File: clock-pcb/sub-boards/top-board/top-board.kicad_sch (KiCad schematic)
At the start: 18 parts, among them J1 Conn_01x07_Socket, U1 BH1750FVI-TR, U3 OPT3004DTSR, U4 SHT4x

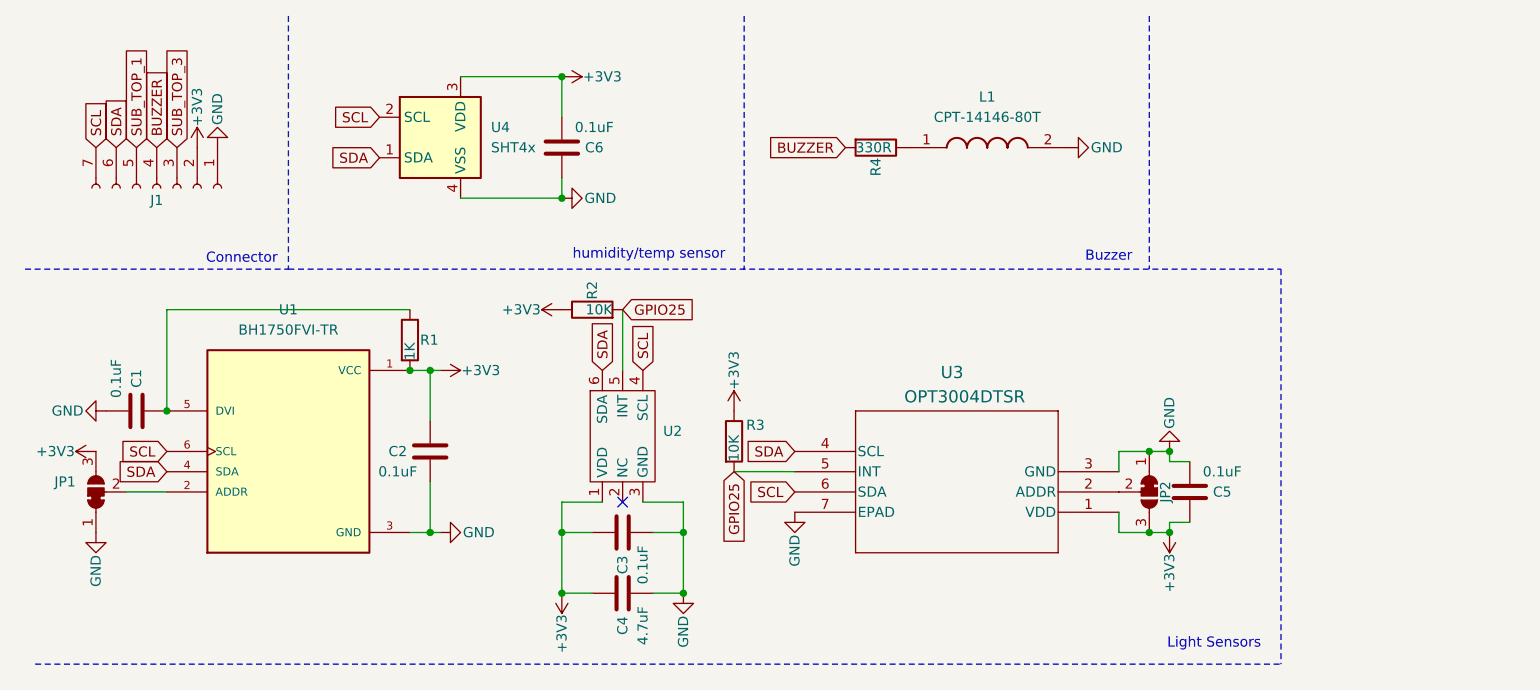
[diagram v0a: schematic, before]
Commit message: routing
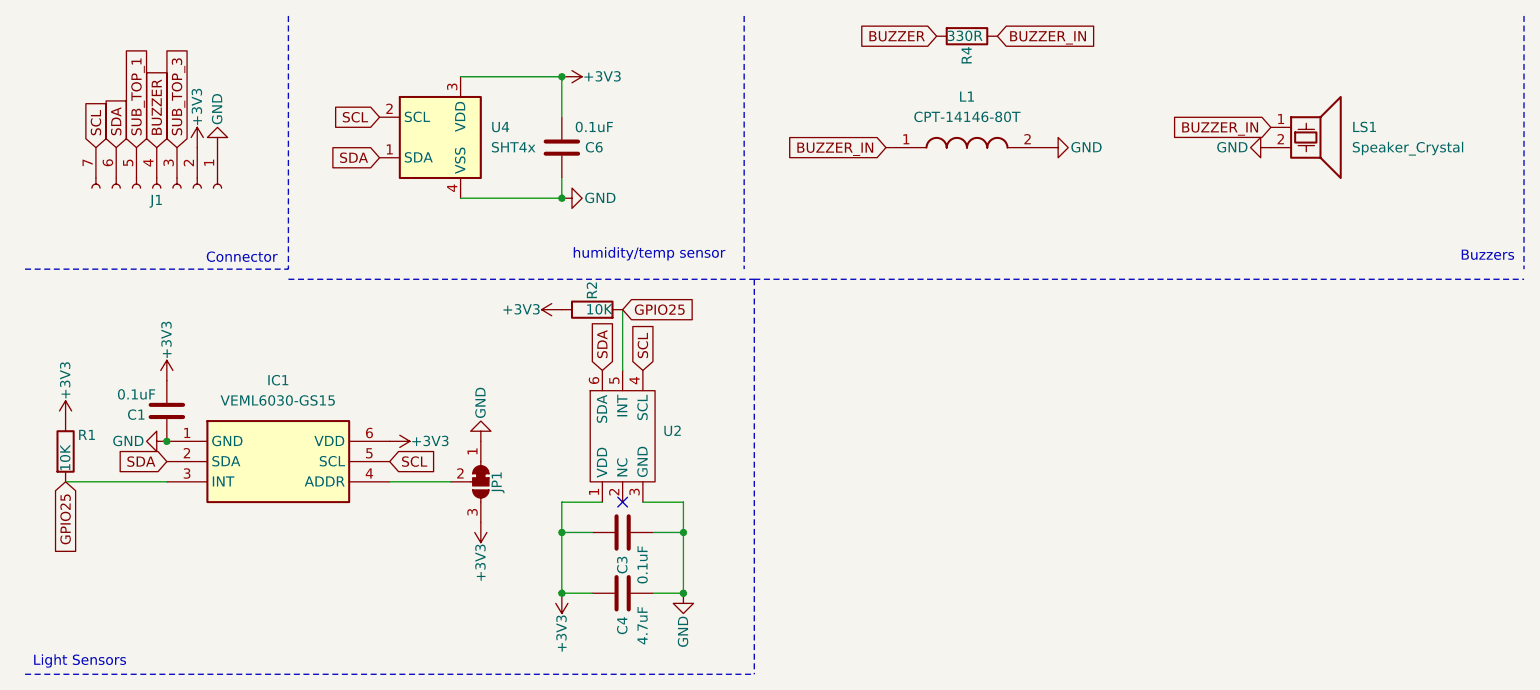
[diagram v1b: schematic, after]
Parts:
- removed C2, C5: 0.1uF, Capacitor_SMD:C_0603_1608Metric, symbol clock:C
- removed JP2: SolderJumper_3_Bridged12, Jumper:SolderJumper-3_P1.3mm_Bridged2Bar12_RoundedPad1.0x1.5mm, symbol clock:SolderJumper_3_Bridged12
- removed R3: 10K, Resistor_SMD:R_0402_1005Metric, symbol clock:R
- removed U1: BH1750FVI-TR, clock:XDCR_BH1750FVI-TR, symbol clock:BH1750FVI-TR
- removed U3: OPT3004DTSR, clock:DNP6_TEX, symbol clock:OPT3004DTSR
- added IC1: VEML6030-GS15, clock:VEML6030GS15, symbol VEML6030-GS15:VEML6030-GS15
- added LS1: Speaker_Crystal, clock:AST0760_MAL, symbol Device:Speaker_Crystal
- R1: value 1K -> 10K
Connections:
- net +3V3: now also C1.2, R1.1, IC1.6 (VDD); no longer R1.2
- net GND: now also C1.1, IC1.1 (GND), LS1.2; no longer C1.2
- net GPIO25: now also R1.2, IC1.3 (INT)
- net SCL: now also IC1.5 (SCL)
- net SDA: now also IC1.2 (SDA)
- net at JP1.2 (C): now also IC1.4 (ADDR)
- net BUZZER_IN: now reaches L1.1, R4.1
- net BUZZER_IN: now also LS1.1
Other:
- note added: "Buzzers"
- note removed: "Buzzer"
- moved on the sheet: L1, R4

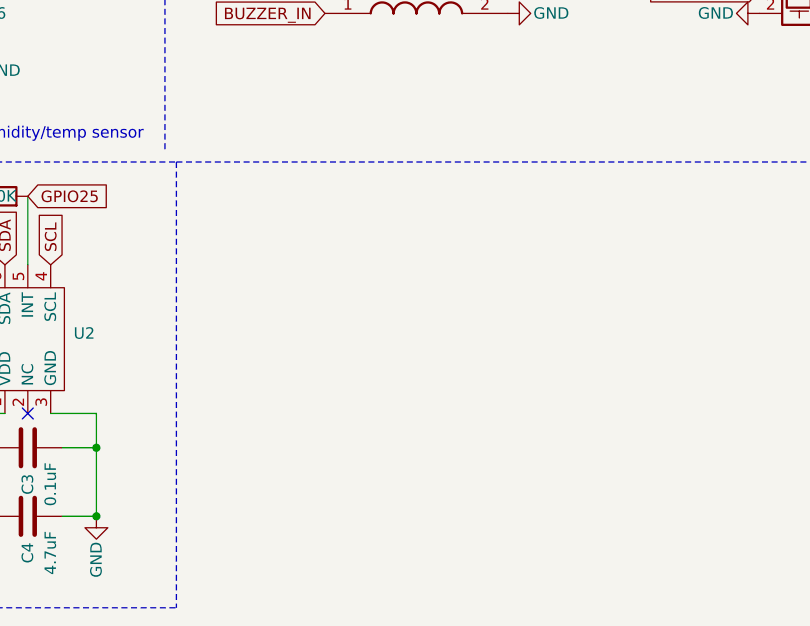
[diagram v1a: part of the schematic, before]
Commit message: touch slider pcb
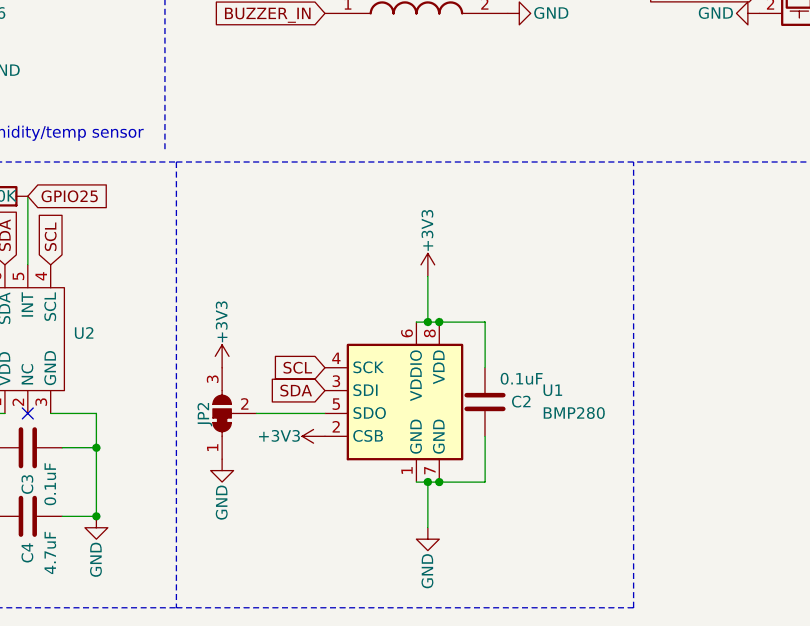
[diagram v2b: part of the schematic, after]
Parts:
- added C2: 0.1uF, Capacitor_SMD:C_0603_1608Metric, symbol clock:C
- added JP2: SolderJumper_3_Bridged12, Jumper:SolderJumper-3_P1.3mm_Bridged2Bar12_RoundedPad1.0x1.5mm, symbol clock:SolderJumper_3_Bridged12
- added U1: BMP280, Package_LGA:Bosch_LGA-8_2x2.5mm_P0.65mm_ClockwisePinNumbering, symbol Sensor_Pressure:BMP280
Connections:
- net +3V3: now also C2.2, JP2.3 (B), U1.2 (CSB), U1.6 (VDDIO), U1.8 (VDD)
- net GND: now also C2.1, JP2.1 (A), U1.1 (GND), U1.7 (GND)
- net SCL: now also U1.4 (SCK)
- net SDA: now also U1.3 (SDI)
- new net: JP2.2 (C), U1.5 (SDO)
